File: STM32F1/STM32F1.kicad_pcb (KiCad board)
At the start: 2 copper layers, 55.9 x 22.9 mm, 40 parts, among them J1 Conn_02x03_Odd_Even, J2 Conn_01x04_Male, J3 10033526-N3212MLF, J4 Conn_01x20_Male, J5 Conn_01x20_Male, SW1 PTS 647 SK38 SMTR2 LFS, U1 RT9193, U2 STM32F103CBTx, Y1 ABL-8.000MHZ-B2‎, Y2 RSM200S-32.768-12.5-10PPM-NPB

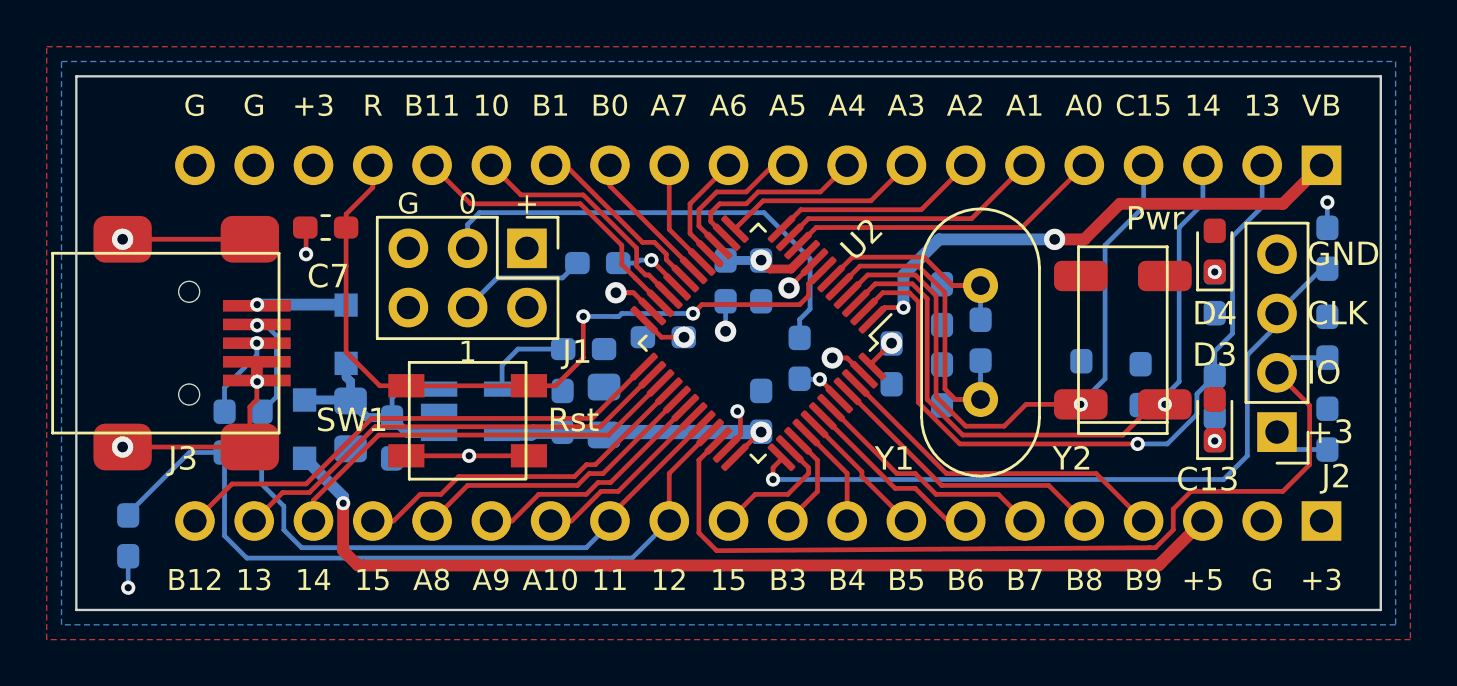
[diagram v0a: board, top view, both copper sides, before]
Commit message: Boards sent to be built.
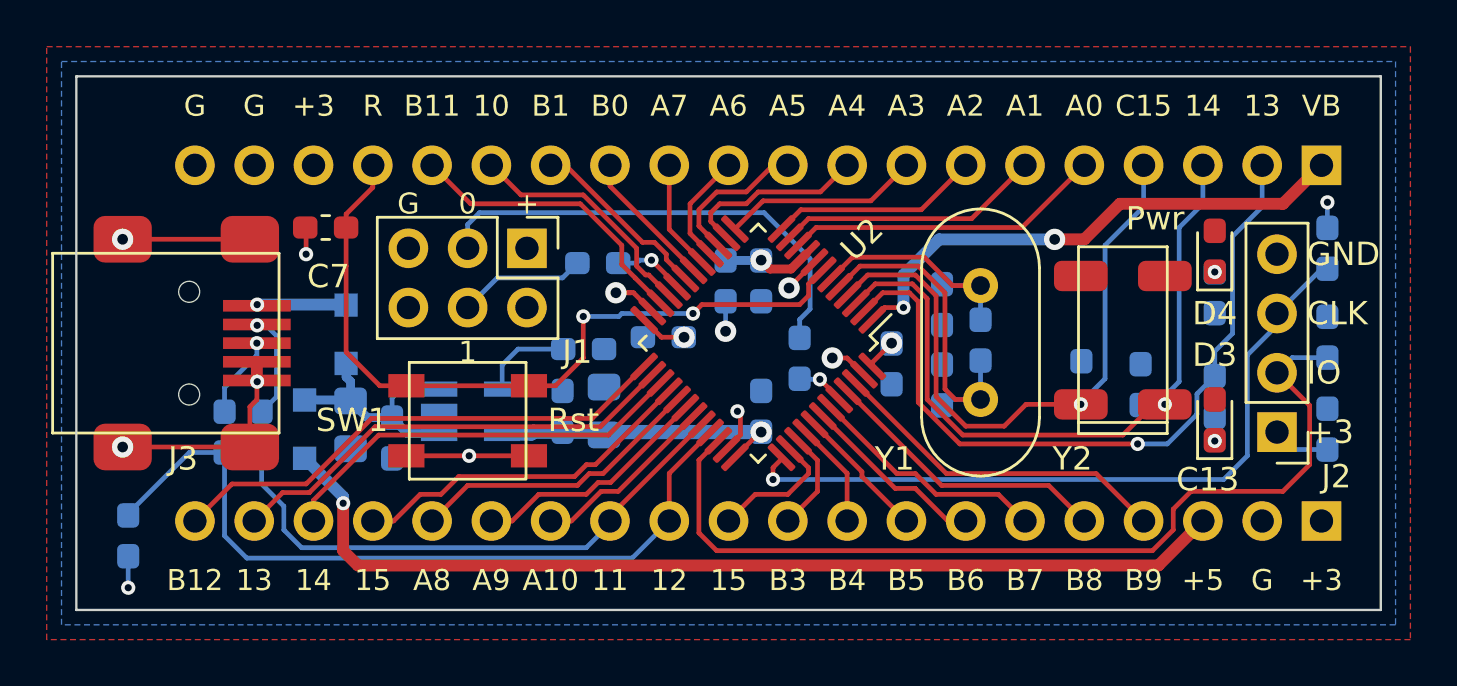
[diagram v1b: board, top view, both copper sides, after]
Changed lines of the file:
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@@
     (thickness 1.6)
     (drawings 58)
-    (tracks 398)
+    (tracks 393)
     (zones 0)
     (modules 40)
@@
   (segment (start 166.878 101.219) (end 166.878 101.219) (width 0.2032) (layer F.Cu) (net 3))
   (via (at 164.211 101.6) (size 0.6096) (drill 0.3048) (layers F.Cu B.Cu) (net 3))
-  (segment (start 160.909 101.727) (end 159.512 101.727) (width 0.2032) (layer B.Cu) (net 3))
-  (segment (start 164.211 101.6) (end 161.163 101.6) (width 0.2032) (layer B.Cu) (net 3))
-  (segment (start 161.036 101.727) (end 160.909 101.727) (width 0.2032) (layer B.Cu) (net 3))
-  (segment (start 161.163 101.6) (end 161.036 101.727) (width 0.2032) (layer B.Cu) (net 3))
   (segment (start 168.783 101.219) (end 164.592 101.219) (width 0.2032) (layer F.Cu) (net 3))
   (segment (start 169.771555 99.749891) (end 169.744109 99.749891) (width 0.2032) (layer F.Cu) (net 3))
@@
   (segment (start 169.744109 99.749891) (end 169.164 100.33) (width 0.2032) (layer F.Cu) (net 3))
   (segment (start 169.164 100.838) (end 168.783 101.219) (width 0.2032) (layer F.Cu) (net 3))
+  (segment (start 164.211 101.6) (end 161.163 101.6) (width 0.2032) (layer B.Cu) (net 3))
+  (segment (start 161.036 101.727) (end 159.512 101.727) (width 0.2032) (layer B.Cu) (net 3))
+  (segment (start 161.163 101.6) (end 161.036 101.727) (width 0.2032) (layer B.Cu) (net 3))
   (via (at 165.608 102.362) (size 0.9144) (drill 0.4572) (layers F.Cu B.Cu) (net 4))
   (via (at 191.389 96.8375) (size 0.6096) (drill 0.3048) (layers F.Cu B.Cu) (net 4))
@@
   (segment (start 167.64 108.712) (end 186.944 108.712) (width 0.2032) (layer B.Cu) (net 8))
   (segment (start 186.944 108.712) (end 187.96 107.696) (width 0.2032) (layer B.Cu) (net 8))
+  (segment (start 189.879 103.491) (end 189.23 104.14) (width 0.2032) (layer B.Cu) (net 9))
+  (segment (start 191.389 103.491) (end 189.879 103.491) (width 0.2032) (layer B.Cu) (net 9))
+  (segment (start 190.627 105.537) (end 189.23 104.14) (width 0.2032) (layer F.Cu) (net 9))
+  (segment (start 165.227 111.76) (end 183.896 111.76) (width 0.2032) (layer F.Cu) (net 9))
+  (segment (start 165.299105 107.050769) (end 164.476074 107.8738) (width 0.2032) (layer F.Cu) (net 9))
+  (segment (start 164.465 110.998) (end 165.227 111.76) (width 0.2032) (layer F.Cu) (net 9))
+  (segment (start 183.896 111.76) (end 184.785 110.871) (width 0.2032) (layer F.Cu) (net 9))
+  (segment (start 164.476074 107.8738) (end 164.465 107.8738) (width 0.2032) (layer F.Cu) (net 9))
+  (segment (start 184.785 110.871) (end 184.785 109.982) (width 0.2032) (layer F.Cu) (net 9))
   (segment (start 190.627 108.077) (end 190.627 105.537) (width 0.2032) (layer F.Cu) (net 9))
   (segment (start 164.465 107.8738) (end 164.465 110.998) (width 0.2032) (layer F.Cu) (net 9))
+  (segment (start 184.785 109.982) (end 185.547 109.22) (width 0.2032) (layer F.Cu) (net 9))
+  (segment (start 185.547 109.22) (end 189.484 109.22) (width 0.2032) (layer F.Cu) (net 9))
   (segment (start 189.484 109.22) (end 190.627 108.077) (width 0.2032) (layer F.Cu) (net 9))
-  (segment (start 165.227 111.76) (end 183.769 111.633) (width 0.2032) (layer F.Cu) (net 9))
-  (segment (start 165.299105 107.050769) (end 164.476074 107.8738) (width 0.2032) (layer F.Cu) (net 9))
-  (segment (start 164.465 110.998) (end 165.227 111.76) (width 0.2032) (layer F.Cu) (net 9))
-  (segment (start 183.769 111.633) (end 184.023 111.633) (width 0.2032) (layer F.Cu) (net 9))
-  (segment (start 185.547 109.22) (end 189.484 109.22) (width 0.2032) (layer F.Cu) (net 9))
-  (segment (start 164.476074 107.8738) (end 164.465 107.8738) (width 0.2032) (layer F.Cu) (net 9))
-  (segment (start 190.627 105.537) (end 189.23 104.14) (width 0.2032) (layer F.Cu) (net 9))
-  (segment (start 184.785 109.982) (end 185.547 109.22) (width 0.2032) (layer F.Cu) (net 9))
-  (segment (start 184.023 111.633) (end 184.785 110.871) (width 0.2032) (layer F.Cu) (net 9))
-  (segment (start 184.785 110.871) (end 184.785 109.982) (width 0.2032) (layer F.Cu) (net 9))
-  (segment (start 189.879 103.491) (end 189.23 104.14) (width 0.2032) (layer B.Cu) (net 9))
-  (segment (start 191.389 103.491) (end 189.879 103.491) (width 0.2032) (layer B.Cu) (net 9))
   (via (at 145.529 102.87) (size 0.6096) (drill 0.3048) (layers F.Cu B.Cu) (net 10))
   (segment (start 145.529 103.391) (end 145.529 102.87) (width 0.2032) (layer B.Cu) (net 10))
@@
   (segment (start 160.655 110.49) (end 160.655 110.28066) (width 0.2032) (layer F.Cu) (net 34))
   (segment (start 147.447 111.633) (end 146.685 110.871) (width 0.2032) (layer B.Cu) (net 34))
+  (segment (start 145.7325 108.9025) (end 145.7325 107.555) (width 0.2032) (layer B.Cu) (net 34))
+  (segment (start 146.685 109.855) (end 145.7325 108.9025) (width 0.2032) (layer B.Cu) (net 34))
+  (segment (start 146.685 110.871) (end 146.685 109.855) (width 0.2032) (layer B.Cu) (net 34))
+  (segment (start 160.655 110.617) (end 159.639 111.633) (width 0.2032) (layer B.Cu) (net 34))
+  (segment (start 160.655 110.49) (end 160.655 110.617) (width 0.2032) (layer B.Cu) (net 34))
   (segment (start 159.639 111.633) (end 147.447 111.633) (width 0.2032) (layer B.Cu) (net 34))
-  (segment (start 160.655 110.49) (end 160.655 110.617) (width 0.2032) (layer B.Cu) (net 34))
-  (segment (start 160.655 110.617) (end 159.639 111.633) (width 0.2032) (layer B.Cu) (net 34))
-  (segment (start 146.685 110.871) (end 146.685 109.855) (width 0.2032) (layer B.Cu) (net 34))
-  (segment (start 146.685 109.855) (end 145.7325 108.9025) (width 0.2032) (layer B.Cu) (net 34))
-  (segment (start 145.7325 108.9025) (end 145.7325 107.555) (width 0.2032) (layer B.Cu) (net 34))
   (segment (start 163.195 108.447766) (end 164.945551 106.697215) (width 0.2032) (layer F.Cu) (net 35))
   (segment (start 163.195 110.49) (end 163.195 108.447766) (width 0.2032) (layer F.Cu) (net 35))
   (segment (start 145.0975 112.0775) (end 144.145 111.125) (width 0.2032) (layer B.Cu) (net 35))
+  (segment (start 161.6075 112.0775) (end 145.0975 112.0775) (width 0.2032) (layer B.Cu) (net 35))
+  (segment (start 144.145 111.125) (end 144.145 107.555) (width 0.2032) (layer B.Cu) (net 35))
   (segment (start 163.195 110.49) (end 161.6075 112.0775) (width 0.2032) (layer B.Cu) (net 35))
-  (segment (start 144.145 111.125) (end 144.145 107.555) (width 0.2032) (layer B.Cu) (net 35))
-  (segment (start 161.6075 112.0775) (end 145.0975 112.0775) (width 0.2032) (layer B.Cu) (net 35))
   (segment (start 142.635 107.555) (end 144.145 107.555) (width 0.2032) (layer B.Cu) (net 35))
   (segment (start 140.335 109.855) (end 142.635 107.555) (width 0.2032) (layer B.Cu) (net 35))
@@
   (segment (start 167.132 99.314) (end 167.513 99.695) (width 0.381) (layer F.Cu) (net 52))
   (segment (start 168.412234 99.695) (end 169.064449 99.042785) (width 0.381) (layer F.Cu) (net 52))
-  (segment (start 186.055 110.49) (end 184.277 112.268) (width 0.508) (layer F.Cu) (net 53))
-  (segment (start 149.225 111.76) (end 149.225 109.728) (width 0.508) (layer F.Cu) (net 53))
-  (segment (start 149.86 112.395) (end 149.225 111.76) (width 0.508) (layer F.Cu) (net 53))
-  (segment (start 150.114 112.395) (end 149.86 112.395) (width 0.508) (layer F.Cu) (net 53))
-  (segment (start 160.655 112.395) (end 150.114 112.395) (width 0.508) (layer F.Cu) (net 53))
-  (segment (start 184.15 112.395) (end 160.655 112.395) (width 0.508) (layer F.Cu) (net 53))
-  (segment (start 184.277 112.268) (end 184.15 112.395) (width 0.508) (layer F.Cu) (net 53))
   (segment (start 149.225 109.728) (end 149.225 109.728) (width 0.508) (layer F.Cu) (net 53))
   (via (at 149.225 109.728) (size 0.6096) (drill 0.3048) (layers F.Cu B.Cu) (net 53))
   (segment (start 149.225 109.454) (end 147.574 107.803) (width 0.508) (layer B.Cu) (net 53))
   (segment (start 149.225 109.728) (end 149.225 109.454) (width 0.508) (layer B.Cu) (net 53))
+  (segment (start 149.86 112.395) (end 149.225 111.76) (width 0.508) (layer F.Cu) (net 53))
+  (segment (start 149.225 111.76) (end 149.225 109.728) (width 0.508) (layer F.Cu) (net 53))
+  (segment (start 186.055 110.49) (end 184.15 112.395) (width 0.508) (layer F.Cu) (net 53))
+  (segment (start 184.15 112.395) (end 149.86 112.395) (width 0.508) (layer F.Cu) (net 53))
   (zone (net 1) (net_name GND) (layer B.Cu) (hatch edge 0.508)
     (connect_pads (clearance 0.1524))
